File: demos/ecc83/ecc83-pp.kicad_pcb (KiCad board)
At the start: 2 copper layers, 15 parts, among them P1 IN, P2 OUT, P3 POWER, P4 CONN_2, U1 ECC81_83

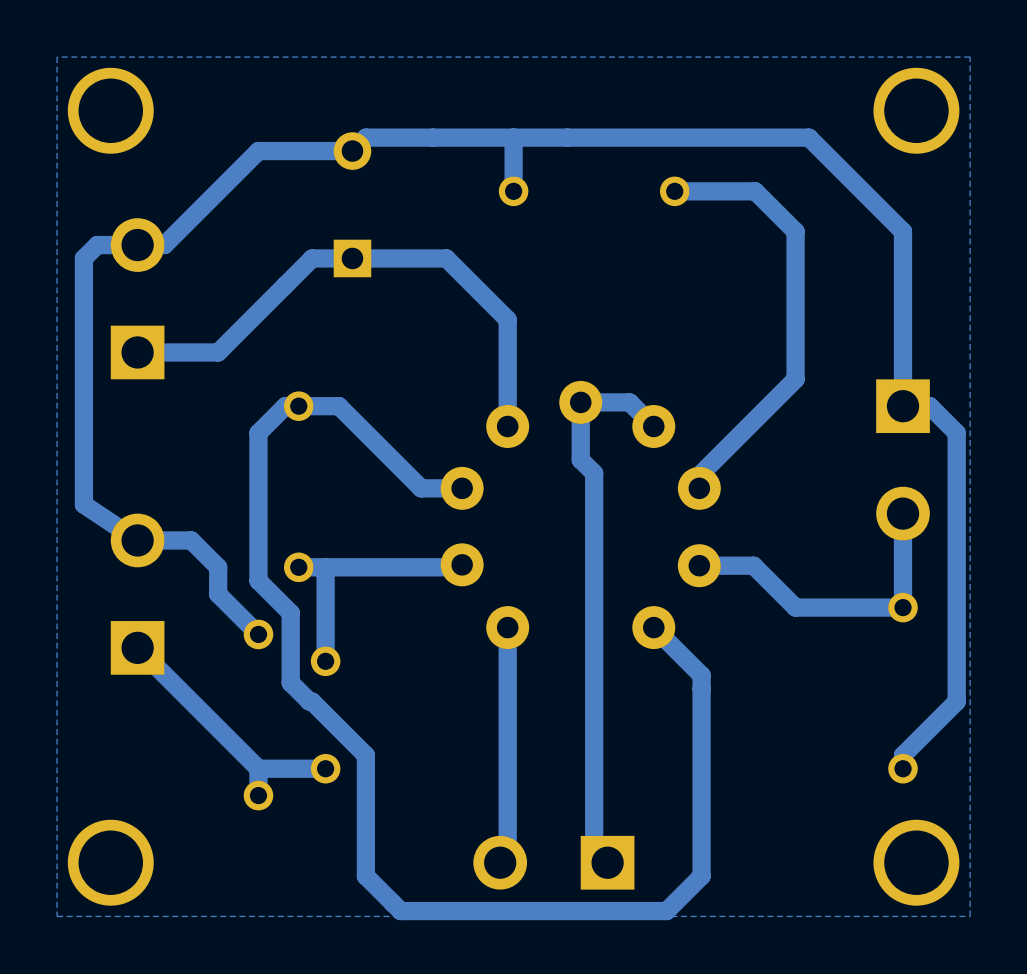
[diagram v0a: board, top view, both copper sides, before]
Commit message: Imported Upstream version 4.0.0~rc1
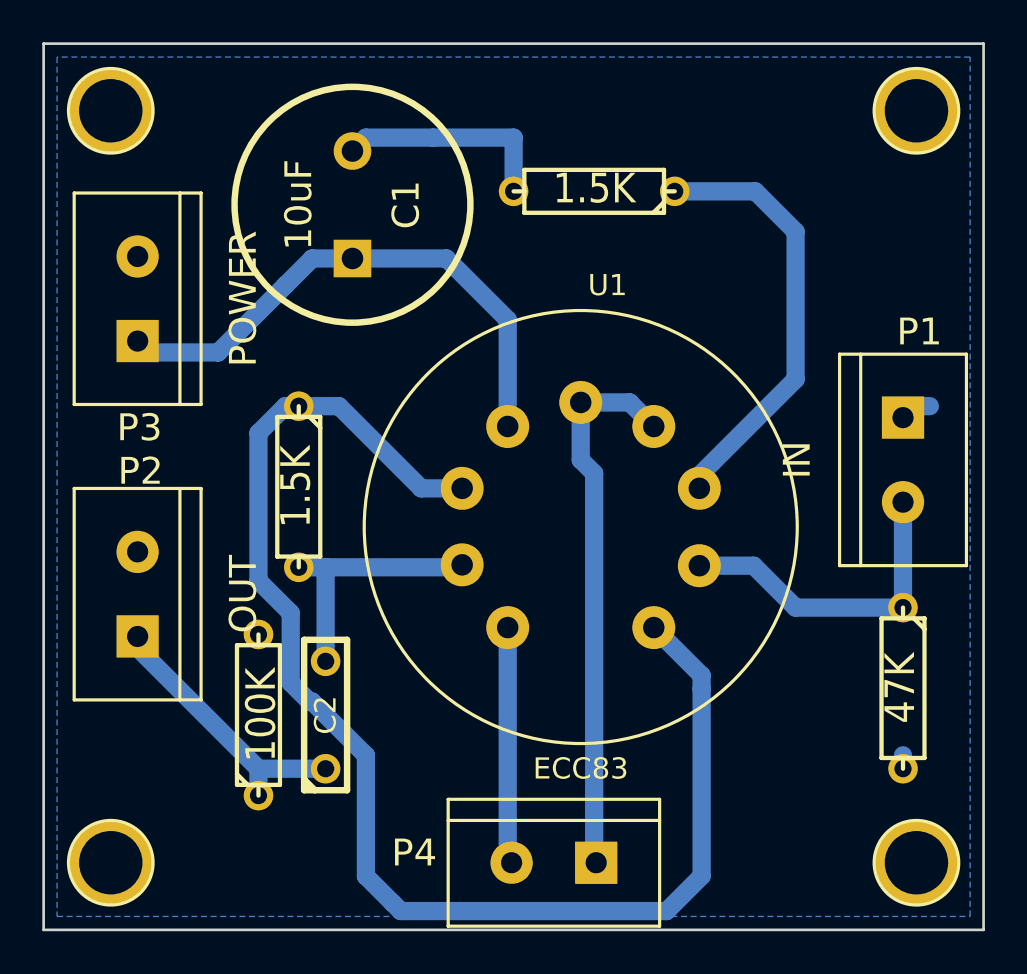
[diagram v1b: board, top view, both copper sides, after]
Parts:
- removed 1PIN (x4): P***, 1pin
- added P5: CONN_1, connect:1pin, F.Cu at (127.0, 94.0)
- added P6: CONN_1, connect:1pin, F.Cu at (165.1, 94.0)
- added P7: CONN_1, connect:1pin, F.Cu at (165.1, 129.5)
- added P8: CONN_1, connect:1pin, F.Cu at (127.0, 129.5)
- C1: footprint C2V10 -> discret:C2V10
- C2: footprint C2 -> discret:C2
- P1, P2, P3, P4: footprint bornier2 -> connect:bornier2
- R1, R2, R3, R4: footprint R3 -> discret:R3
- U1: value ECC81_83 -> ECC83; footprint ECC-83-1 -> Valves:VALVE-ECC-83-1
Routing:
- net GND: track 96.7 -> 12.3 mm
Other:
- board outline added: 44.5 x 41.9 mm
- rule pad_to_mask_clearance: 0.254 -> 0.1
